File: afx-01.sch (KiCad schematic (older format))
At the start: 10 parts, among them P1 CONN_02X05, P2 CONN_02X05, U1 ADA_SSD1306_I2C, U2 Teensy_3.1, U4 MicroSD_Adapter, U5 SSD1306

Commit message: BIG UPDATE! omg so big
New boards and other things.. jeesh it sbeen too long since the last update
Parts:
- removed P2: CONN_02X05, ab2_header:AB2_HDR_M05-2V, symbol CONN_02X05
- removed U5: SSD1306, afx-01:SSD1306_XL, symbol SSD1306
- added P?: CONN_02X05, ab2_header:AB2_HDR_M05-2V, symbol CONN_02X05
- added U?: MCP1703, symbol MCP1703
- U1: footprint afx-01:SSD1306 -> Zetaohm:SSD1306
- U2: footprint afx-01:Teensy3.1 -> Zetaohm:Teensy3.1
- U4: footprint afx-01:MicroSD -> Zetaohm:MicroSD
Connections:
- net labels added: +3V3, +5V, CV_IN1, CV_IN2, CV_IN3, CV_IN4, DAC_CS, DAC_SDO, DISP_RESET, ENC1A, ENC1B, ENC2A, ENC2B, GATE_IN1, GATE_IN2, GATE_IN3, GATE_IN4, GNDA, LED_DIN, MIDI_IN_EXTERNAL, MIDI_OUT_EXTERNAL, MIDI_OUT_INTERNAL, MISO, MOSI, SCL0, SCL1, SCLK, SDA0, SDA1, SD_CS, SPARE_ANALOG1, VDD, VSS
- net labels removed: 10, 11, 12, 13, 15, 20, 22, 24, 25, 26, 29, 3, 30, 4, 5, 6, 9, AGND, VCC, VIN
- wire segments 110 -> 122
- no-connect marks 22 -> 19
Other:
- note added: "5V VOLTAGE REGULATOR"
- note added: "AUX CONNECTOR"
- note added: "EXTERNAL POWER BUS"
- note added: "I2C PULLUP RESISTORS"
- note added: "ZETAOHM AFX-01"
- moved on the sheet: P1, R16, R17, R18, R19, U1, U2, U4

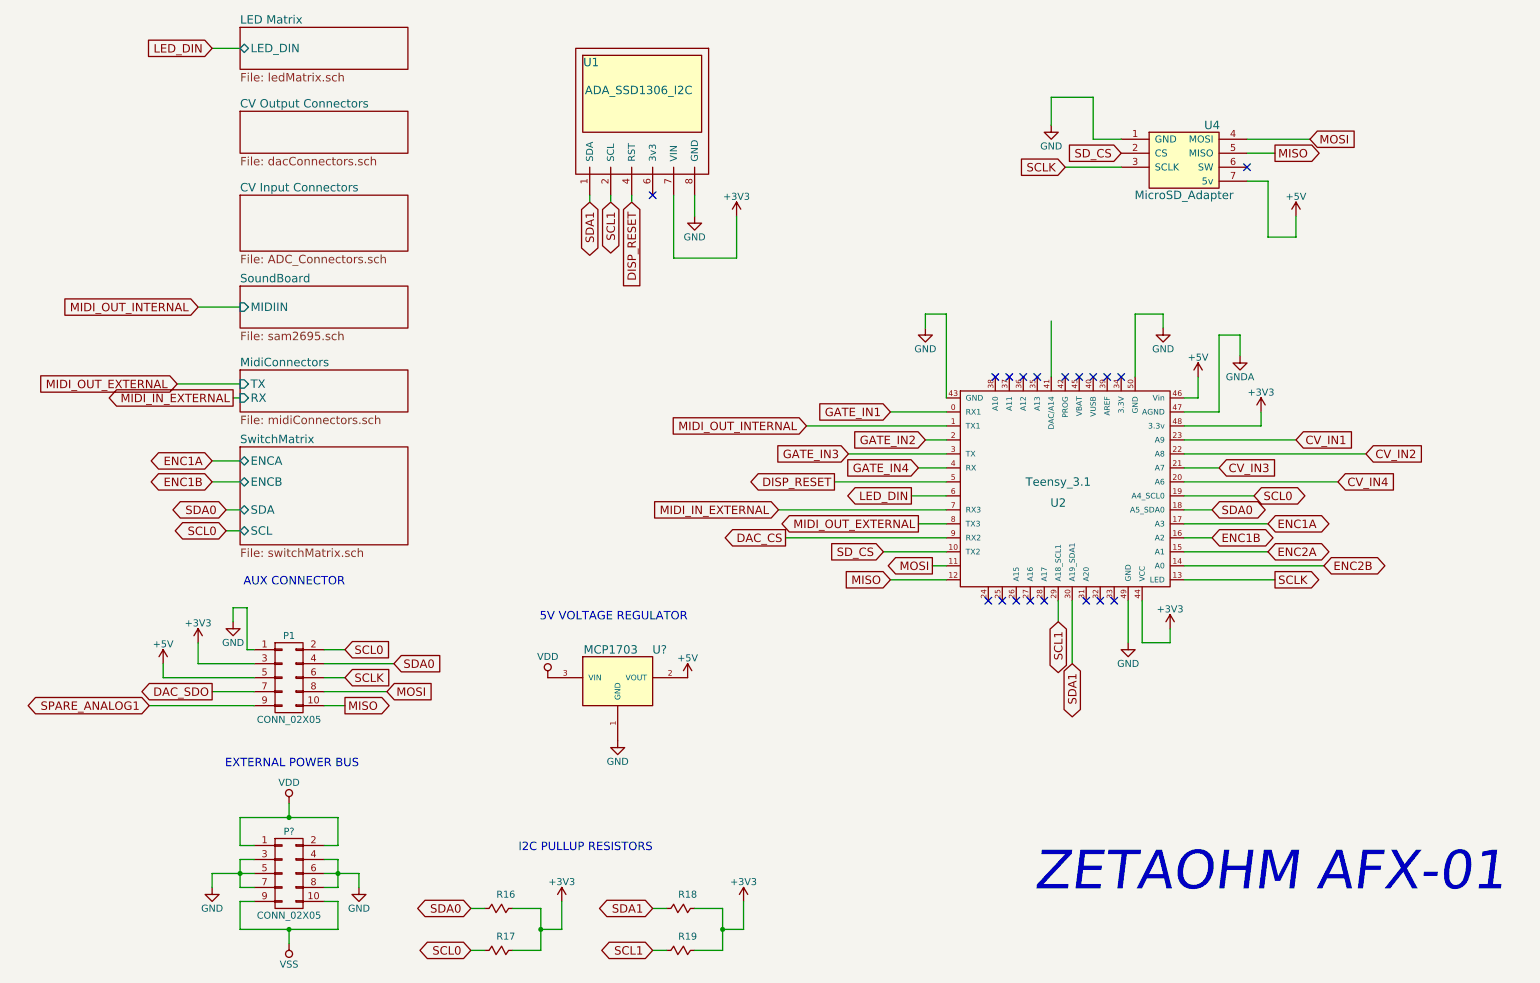
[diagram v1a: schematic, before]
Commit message: UPDATEUPDATES!!!
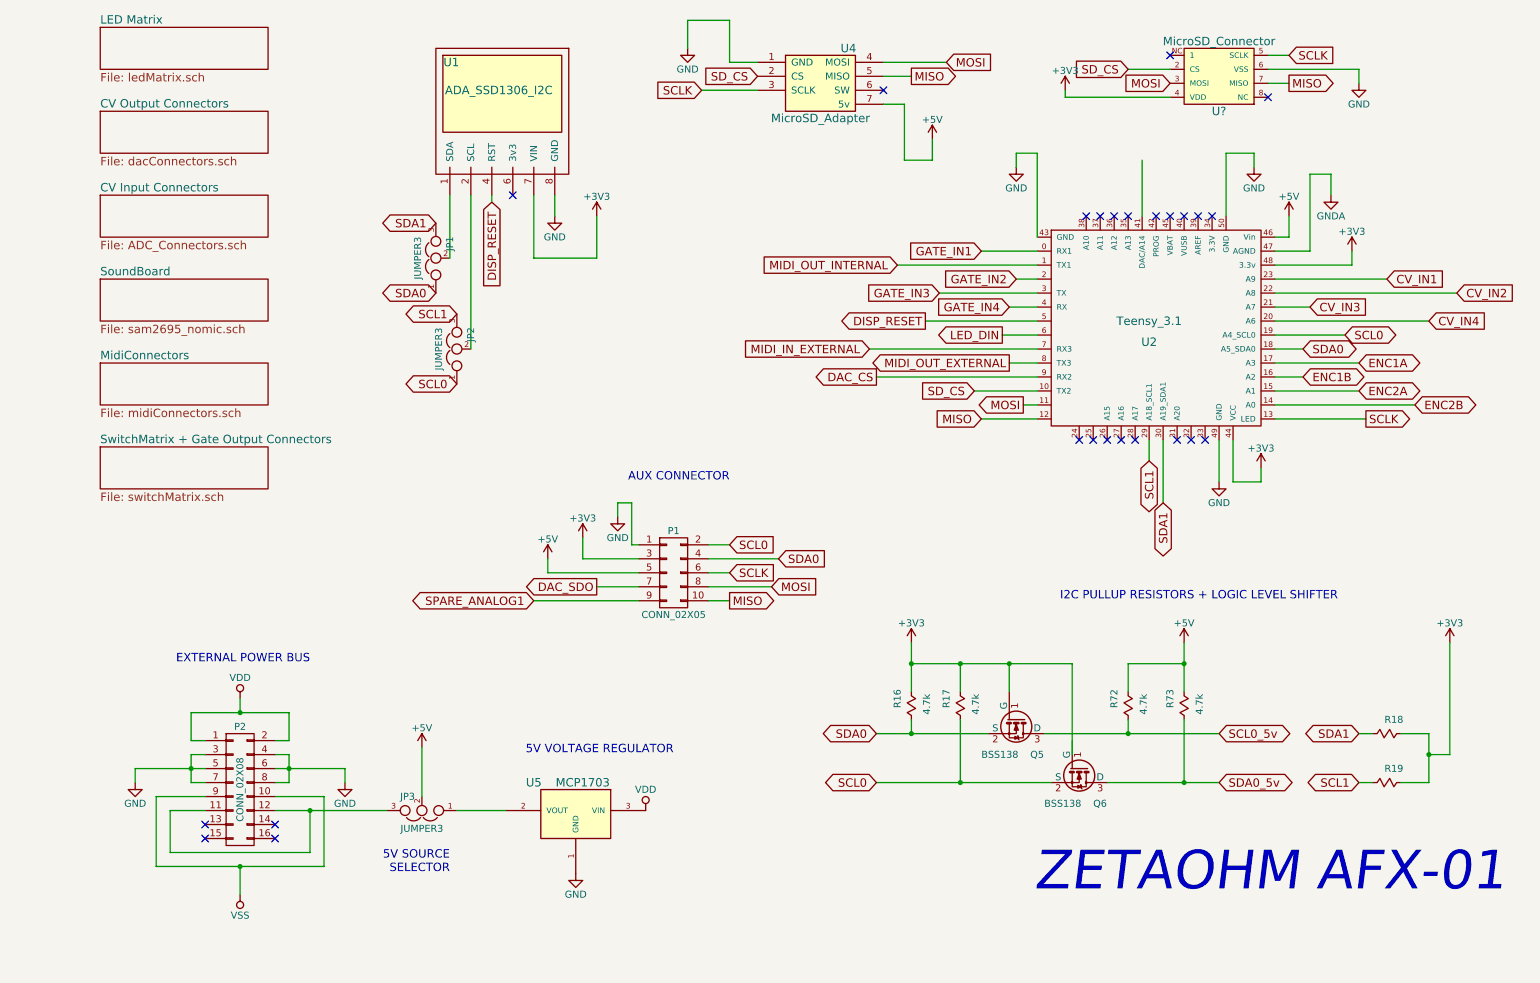
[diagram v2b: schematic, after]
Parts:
- removed P?: CONN_02X05, ab2_header:AB2_HDR_M05-2V, symbol CONN_02X05
- added JP1, JP2, JP3: JUMPER3, Zetaohm:Jumper_3way, symbol JUMPER3
- added P2: CONN_02X08, Pin_Headers:Pin_Header_Angled_2x08, symbol CONN_02X08
- added Q5, Q6: BSS138, Housings_SOT-23_SOT-143_TSOT-6:SOT-23, symbol BSS138
- added R72, R73: 4.7k, Resistors_SMD:R_0805_HandSoldering, symbol Resistor
- added U?: MicroSD_Connector, Zetaohm:AMPHENOL_MICROSD, symbol MicroSD_Connector
- U2: footprint Zetaohm:Teensy3.1 -> Zetaohm:Teensy3.1_Min_I2C2
- U5: renamed from U?; footprint (none) -> Housings_SOT-23_SOT-143_TSOT-6:SOT-23_Handsoldering
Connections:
- net +3V3: now also Q5.1 (G), U?.4 (VDD)
- net +5V: now also JP3.2, R72.2, R73.2; no longer U5.2 (VOUT)
- net GND: now also P2.3 (P3), P2.4 (P4), P2.5 (P5), P2.6 (P6), P2.7 (P7), P2.8 (P8), U?.6 (VSS)
- net MISO: now also U?.7 (MISO)
- net MOSI: now also U?.3 (MOSI)
- net SCL0: now also JP2.1, Q6.2 (S)
- net SCL1: now also JP2.3; no longer U1.2 (SCL)
- net SCLK: now also U?.5 (SCLK)
- net SDA0: now also JP1.1, Q5.2 (S)
- net SDA1: now also JP1.3; no longer U1.1 (SDA)
- net SD_CS: now also U?.2 (CS)
- net VDD: now also P2.1 (P1), P2.2 (P2)
- net VSS: now also P2.10 (P10), P2.9 (P9)
- new net: JP1.2, U1.1 (SDA)
- new net: JP2.2, U1.2 (SCL)
- new net: JP3.1, U5.2 (VOUT)
- new net: JP3.3, P2.11 (P11), P2.12 (P12)
- new net SCL0_5v: Q5.3 (D), R72.1
- new net SDA0_5v: Q6.3 (D), R73.1
- no-connect marks 19 -> 25
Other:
- note added: "5V SOURCE\nSELECTOR"
- note added: "I2C PULLUP RESISTORS + LOGIC LEVEL SHIFTER"
- note removed: "I2C PULLUP RESISTORS"
- moved on the sheet: P1, R16, R17, R18, R19, U1, U2, U4, U5
